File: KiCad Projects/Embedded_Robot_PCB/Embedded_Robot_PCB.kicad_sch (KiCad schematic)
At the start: 7 parts, among them U1 STM32F103RCTx

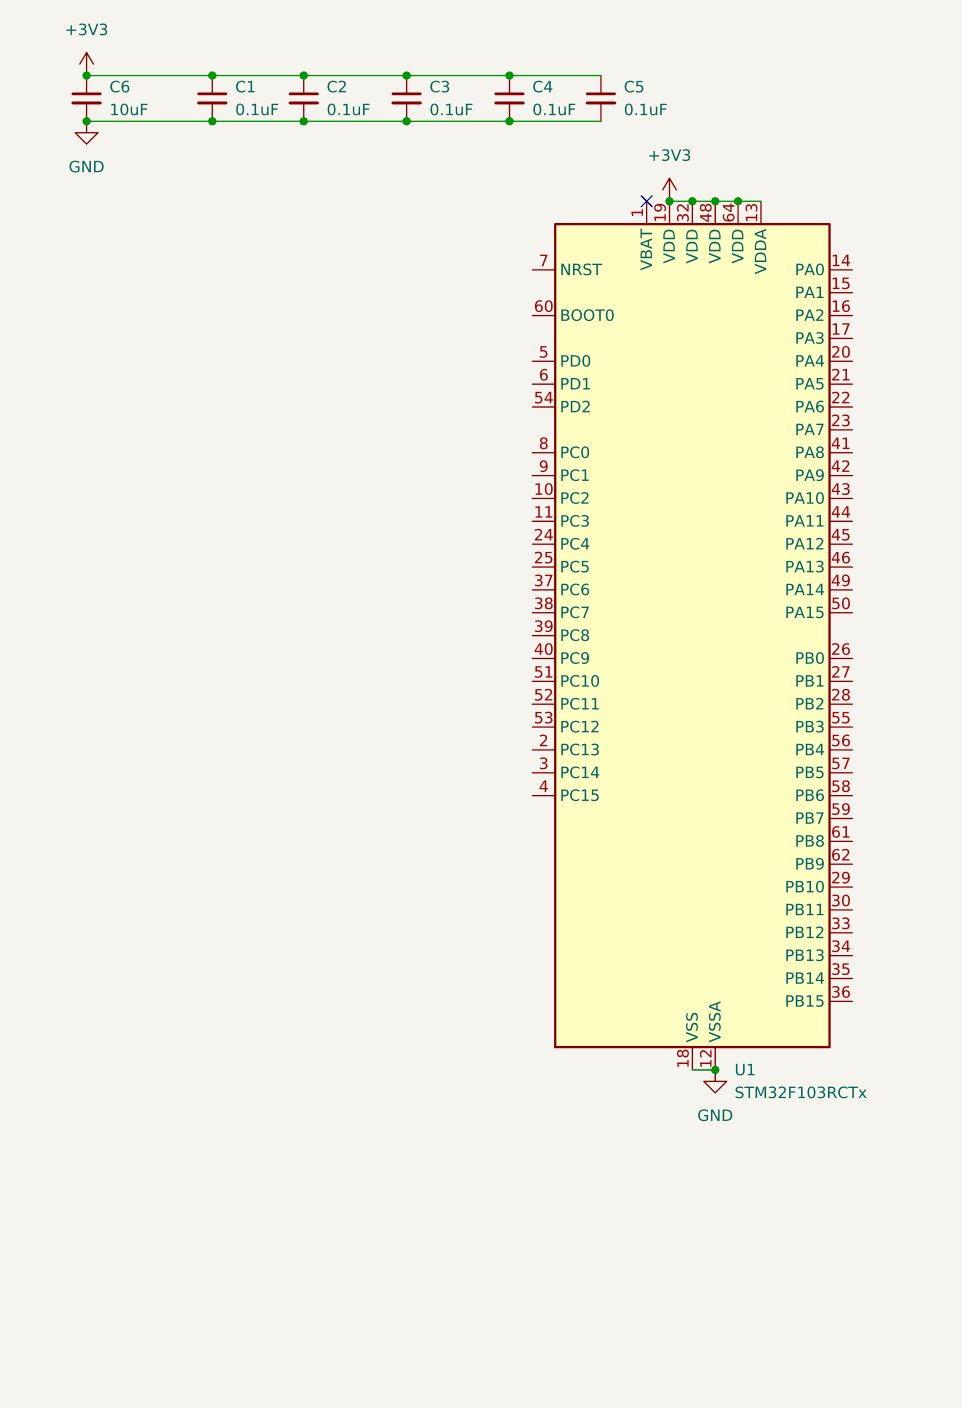
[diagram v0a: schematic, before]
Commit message: 4/24 Inclass Work
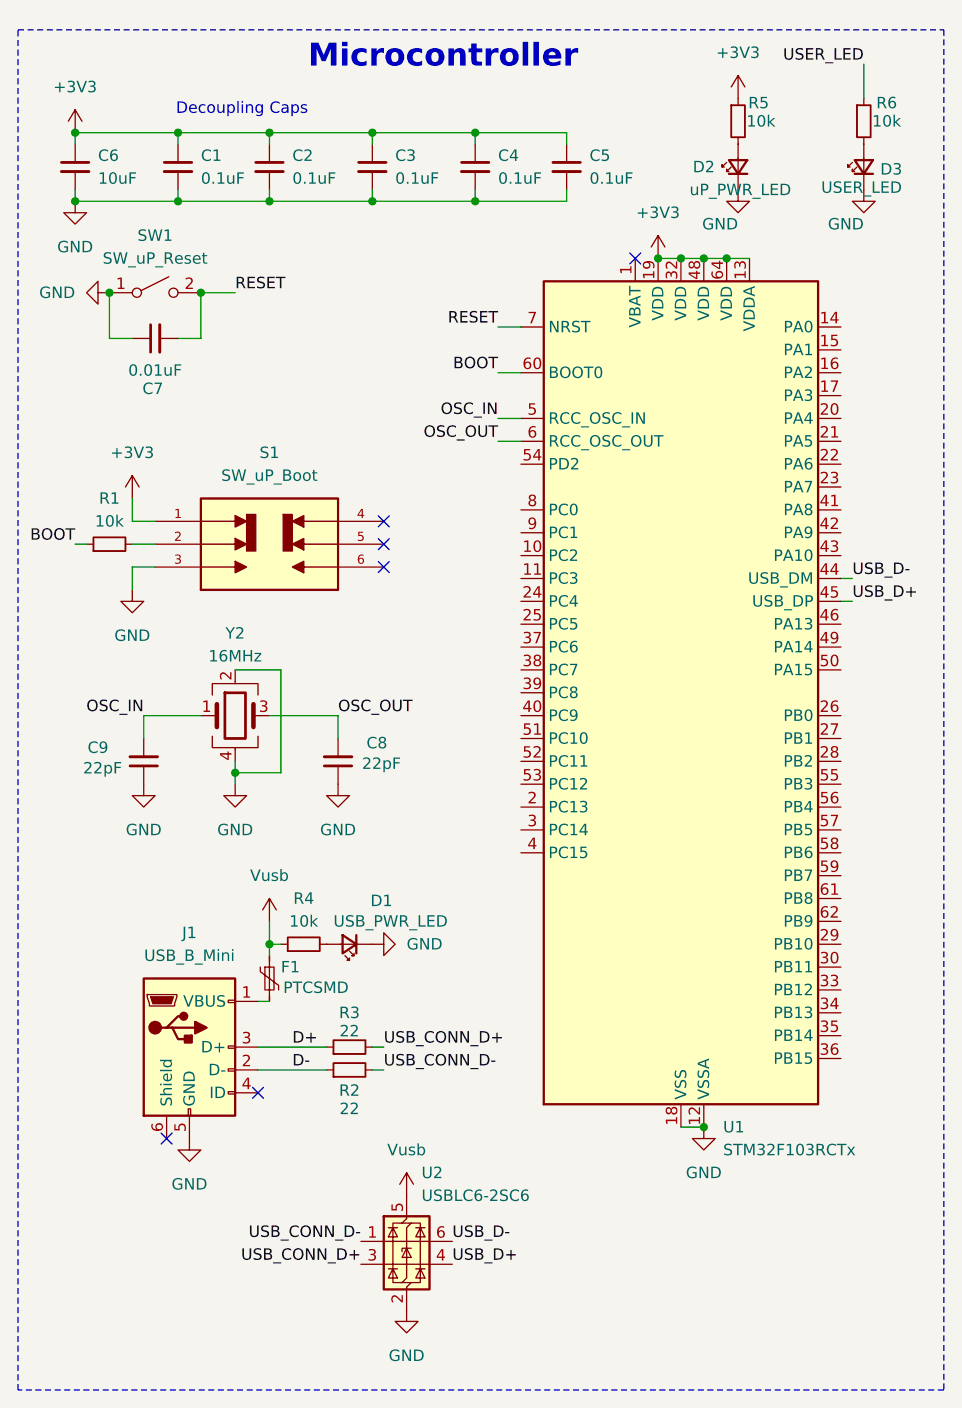
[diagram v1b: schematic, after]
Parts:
- added C7: 0.01uF, Capacitor_SMD:C_0805_2012Metric_Pad1.18x1.45mm_HandSolder, symbol Device:C_Small
- added C8, C9: 22pF, Capacitor_SMD:C_0805_2012Metric_Pad1.18x1.45mm_HandSolder, symbol Device:C_Small
- added D1: USB_PWR_LED, LED_SMD:LED_0805_2012Metric_Pad1.15x1.40mm_HandSolder, symbol Device:LED_Small
- added D2: uP_PWR_LED, LED_SMD:LED_0805_2012Metric_Pad1.15x1.40mm_HandSolder, symbol Device:LED_Small
- added D3: USER_LED, LED_SMD:LED_0805_2012Metric_Pad1.15x1.40mm_HandSolder, symbol Device:LED_Small
- added F1: PTCSMD, Fuse:Fuse_0805_2012Metric_Pad1.15x1.40mm_HandSolder, symbol Device:Polyfuse_Small
- added J1: USB_B_Mini, Connector_USB:USB_Mini-B_Lumberg_2486_01_Horizontal, symbol Connector:USB_B_Mini
- added R1, R4, R5, R6: 10k, Resistor_SMD:R_0805_2012Metric_Pad1.20x1.40mm_HandSolder, symbol Device:R_Small
- added R2, R3: 22, Resistor_SMD:R_0805_2012Metric_Pad1.20x1.40mm_HandSolder, symbol Device:R_Small
- added S1: SW_uP_Boot, SW_uP_Boot:SW_JS202011SCQN, symbol SW_uP_Boot:JS202011SCQN
- added SW1: SW_uP_Reset, SW_uP_Reset:SW_uP_Reset, symbol Switch:SW_SPST
- added U2: USBLC6-2SC6, Package_TO_SOT_SMD:SOT-23-6, symbol Power_Protection:USBLC6-2SC6
- added Y2: 16MHz, Crystal:Crystal_SMD_Abracon_ABM8G-4Pin_3.2x2.5mm, symbol Device:Crystal_GND24
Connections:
- net +3V3: now also R5.1, S1.1
- net GND: now also C7.1, C8.1, C9.1, D1.1 (K), D2.1 (K), D3.1 (K), J1.5 (GND), S1.3, SW1.1 (A), U2.2 (GND), Y2.2, Y2.4
- net USB_D-: now reaches U1.44 (PA11)
- net USB_D-: now also U2.6 (I/O1)
- net USB_D+: now reaches U1.45 (PA12)
- net USB_D+: now also U2.4 (I/O2)
- net OSC_IN: now reaches U1.5 (PD0)
- net OSC_IN: now also C9.2, Y2.1
- net OSC_OUT: now reaches U1.6 (PD1)
- net OSC_OUT: now also C8.2, Y2.3
- net BOOT: now reaches U1.60 (BOOT0)
- net BOOT: now also R1.1
- net RESET: now reaches U1.7 (NRST)
- net RESET: now also C7.2, SW1.2 (B)
- new net: D2.2 (A), R5.2
- new net: F1.2, J1.1 (VBUS)
- new net: R1.2, S1.2
- new net: D3.2 (A), R6.2
- new net: D1.2 (A), R4.2
- new net D+: J1.3 (D+), R3.1
- new net D-: J1.2 (D-), R2.1
- new net USB_CONN_D+: R3.2, U2.3 (I/O2)
- new net USB_CONN_D-: R2.2, U2.1 (I/O1)
- new net USER_LED: R6.1
- new net Vusb: F1.1, R4.1, U2.5 (VBUS)
- no-connect marks 1 -> 6
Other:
- note added: "Decoupling Caps"
- note added: "Microcontroller"
- moved on the sheet: C1, C2, C3, C4, C5, C6, U1
